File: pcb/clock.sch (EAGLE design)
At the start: 50 parts, among them K1 JS-M1-9V-4, K2 JS-M1-9V-4, Q1 BC447, Q2 BC447, Q3 BC447, Q4 BC447, Q5 BC447, Q6 BC447, Q8 CSM-7X-DU, Q9 MC-306, U1 ATMEGA328P-AU, U2 PCF8563T/F4

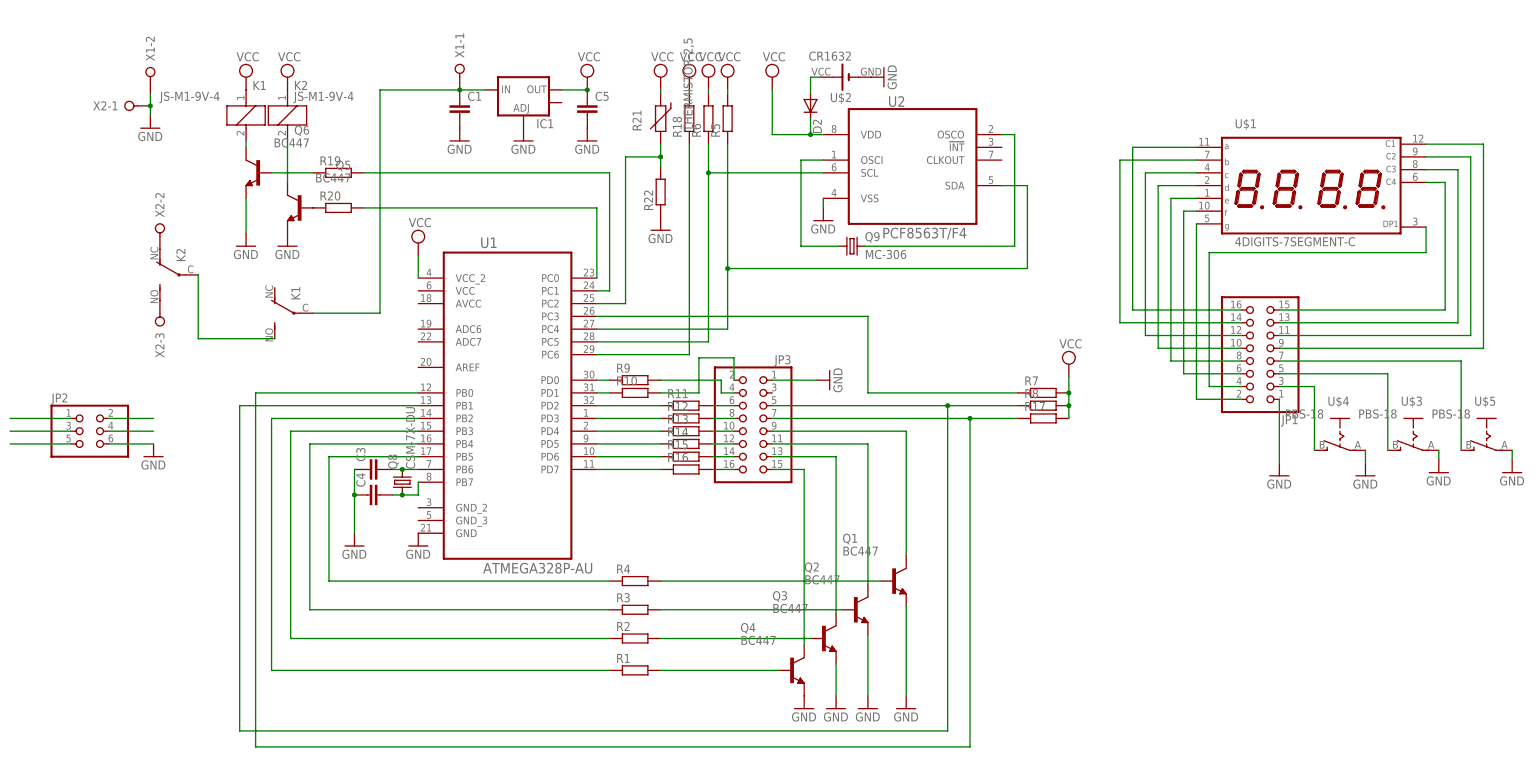
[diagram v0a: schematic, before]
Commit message: some small things
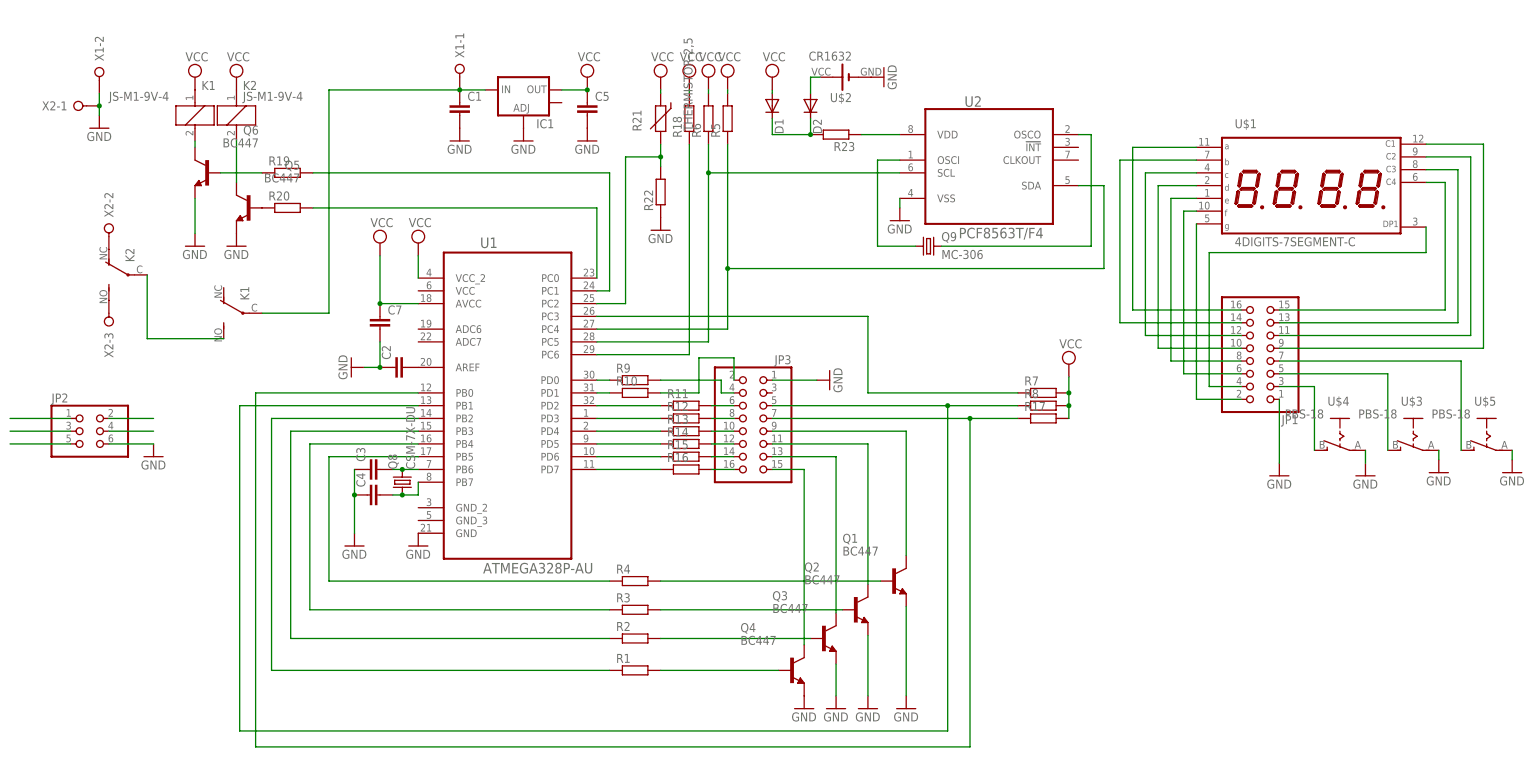
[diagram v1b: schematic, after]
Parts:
- added C2: (no value), rcl:C-EUC1206
- added C7: (no value), rcl:C-EU025-040X050
- added D1: (no value), diode:DIODE-SOD80C
- added R23: (no value), rcl:R-EU_R1206
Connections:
- new net N$66: C2.2, U1.AREF
- new net N$67: D1.C, D2.C, R23.2
- new net N$68: R23.1, U2.VDD
- net GND: now also C2.1, C7.2
- net VCC: now also C7.1, D1.A, U1.AVCC; no longer D2.C, U2.VDD
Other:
- moved on the sheet: K1, K2, Q5, Q6, Q9, R19, R20, U2, X1-2, X2-1, X2-2, X2-3
